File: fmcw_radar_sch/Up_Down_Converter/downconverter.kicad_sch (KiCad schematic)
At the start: 19 parts, among them J11 Conn_Coaxial, J12 Conn_Coaxial, J13 Conn_Coaxial, J14 Conn_01x05_Pin, J6 Conn_Coaxial, U1 ADAR2004ACCZ

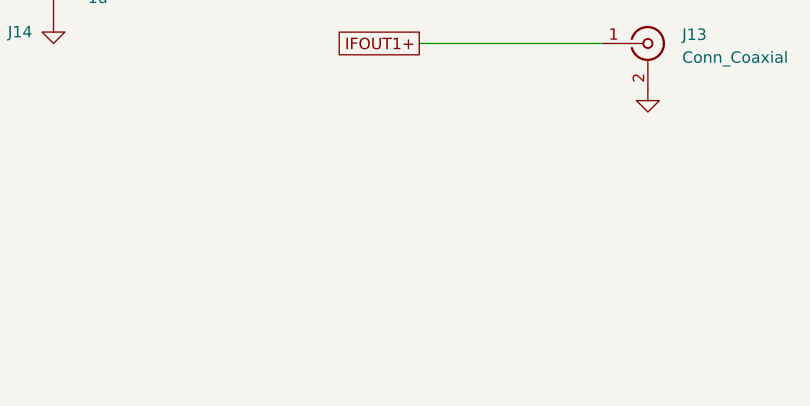
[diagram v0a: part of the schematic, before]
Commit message: changes
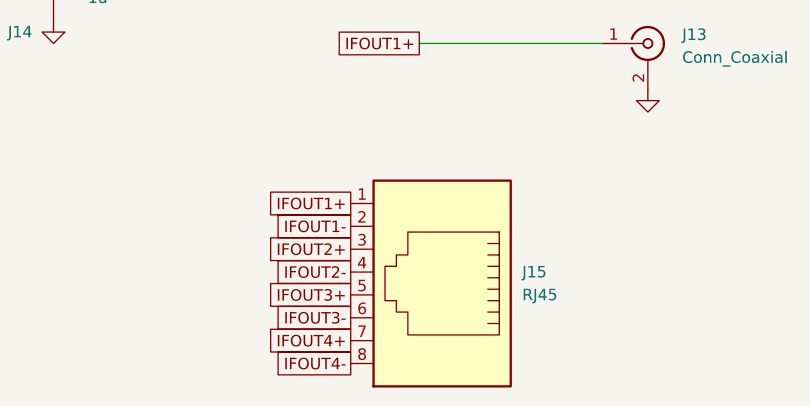
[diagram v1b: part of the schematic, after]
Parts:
- added J15: RJ45, Connector_RJ:RJ45_Amphenol_54602-x08_Horizontal, symbol Connector:RJ45
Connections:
- net IFOUT1+: now also J15.1
- net IFOUT1-: now also J15.2
- net IFOUT2+: now also J15.3
- net IFOUT2-: now also J15.4
- net IFOUT3+: now also J15.5
- net IFOUT3-: now also J15.6
- net IFOUT4+: now also J15.7
- net IFOUT4-: now also J15.8
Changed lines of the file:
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@@
 		)
 	)
+	(global_label "IFOUT4+"
+		(shape passive)
+		(at 208.28 148.59 180)
+		(effects
+			(font
+				(size 1.27 1.27)
+			)
+			(justify right)
+		)
+		(property "Intersheetrefs" "${INTERSHEET_REFS}"
+			(at 208.28 148.59 0)
+			(effects
+				(font
+					(size 1.27 1.27)
+				)
+				(hide yes)
+			)
+		)
+	)
 	(global_label "IFOUT1+"
 		(shape passive)
@@
 		)
 	)
+	(global_label "IFOUT1-"
+		(shape passive)
+		(at 208.28 135.89 180)
+		(effects
+			(font
+				(size 1.27 1.27)
+			)
+			(justify right)
+		)
+		(property "Intersheetrefs" "${INTERSHEET_REFS}"
+			(at 208.28 135.89 0)
+			(effects
+				(font
+					(size 1.27 1.27)
+				)
+				(hide yes)
+			)
+		)
+	)
 	(global_label "RFIN3+"
 		(shape passive)
@@
 		)
 	)
+	(global_label "IFOUT4-"
+		(shape passive)
+		(at 208.28 151.13 180)
+		(effects
+			(font
+				(size 1.27 1.27)
+			)
+			(justify right)
+		)
+		(property "Intersheetrefs" "${INTERSHEET_REFS}"
+			(at 208.28 151.13 0)
+			(effects
+				(font
+					(size 1.27 1.27)
+				)
+				(hide yes)
+			)
+		)
+	)
 	(global_label "RFIN2-"
 		(shape passive)
@@
 		)
 	)
+	(global_label "IFOUT2+"
+		(shape passive)
+		(at 208.28 138.43 180)
+		(effects
+			(font
+				(size 1.27 1.27)
+			)
+			(justify right)
+		)
+		(property "Intersheetrefs" "${INTERSHEET_REFS}"
+			(at 208.28 138.43 0)
+			(effects
+				(font
+					(size 1.27 1.27)
+				)
+				(hide yes)
+			)
+		)
+	)
 	(global_label "IFOUT4-"
 		(shape passive)
@@
 		)
 	)
+	(global_label "IFOUT1+"
+		(shape passive)
+		(at 208.28 133.35 180)
+		(effects
+			(font
+				(size 1.27 1.27)
+			)
+			(justify right)
+		)
+		(property "Intersheetrefs" "${INTERSHEET_REFS}"
+			(at 208.28 133.35 0)
+			(effects
+				(font
+					(size 1.27 1.27)
+				)
+				(hide yes)
+			)
+		)
+	)
 	(global_label "IFOUT1-"
 		(shape passive)
@@
 		)
 	)
+	(global_label "IFOUT3+"
+		(shape passive)
+		(at 208.28 143.51 180)
+		(effects
+			(font
+				(size 1.27 1.27)
+			)
+			(justify right)
+		)
+		(property "Intersheetrefs" "${INTERSHEET_REFS}"
+			(at 208.28 143.51 0)
+			(effects
+				(font
+					(size 1.27 1.27)
+				)
+				(hide yes)
+			)
+		)
+	)
 	(global_label "RFIN3-"
 		(shape passive)
@@
 		)
 	)
+	(global_label "IFOUT3-"
+		(shape passive)
+		(at 208.28 146.05 180)
+		(effects
+			(font
+				(size 1.27 1.27)
+			)
+			(justify right)
+		)
+		(property "Intersheetrefs" "${INTERSHEET_REFS}"
+			(at 208.28 146.05 0)
+			(effects
+				(font
+					(size 1.27 1.27)
+				)
+				(hide yes)
+			)
+		)
+	)
 	(global_label "IFOUT2-"
 		(shape passive)
@@
 		)
 	)
+	(global_label "IFOUT2-"
+		(shape passive)
+		(at 208.28 140.97 180)
+		(effects
+			(font
+				(size 1.27 1.27)
+			)
+			(justify right)
+		)
+		(property "Intersheetrefs" "${INTERSHEET_REFS}"
+			(at 208.28 140.97 0)
+			(effects
+				(font
+					(size 1.27 1.27)
+				)
+				(hide yes)
+			)
+		)
+	)
 	(global_label "VPOS4R"
 		(shape input)
@@
 					(unit 1)
 				)
+			)
+		)
+	)
+	(symbol
+		(lib_id "Connector:RJ45")
+		(at 218.44 140.97 180)
+		(unit 1)
+		(exclude_from_sim no)
+		(in_bom yes)
+		(on_board yes)
+		(dnp no)
+		(fields_autoplaced yes)
+		(property "Reference" "J15"
+			(at 227.33 140.9699 0)
+			(effects
+				(font
+					(size 1.27 1.27)
+				)
+				(justify right)
+			)
+		)
+		(property "Value" "RJ45"
+			(at 227.33 143.5099 0)
+			(effects
+				(font
+					(size 1.27 1.27)
+				)
+				(justify right)
+			)
+		)
+		(property "Footprint" "Connector_RJ:RJ45_Amphenol_54602-x08_Horizontal"
+			(at 218.44 141.605 90)
+			(effects
+				(font
+					(size 1.27 1.27)
+				)
+				(hide yes)
+			)
+		)
+		(property "Datasheet" "~"
+			(at 218.44 141.605 90)
+			(effects
+				(font
+					(size 1.27 1.27)
+				)
+				(hide yes)
+			)
+		)
+		(property "Description" "RJ connector, 8P8C (8 positions 8 connected)"
+			(at 218.44 140.97 0)
+			(effects
+				(font
+					(size 1.27 1.27)
+				)
+				(hide yes)
+			)
+		)
+		(pin "2"
+		)
+		(pin "6"
+		)
+		(pin "8"
+		)
+		(pin "7"
+		)
+		(pin "4"
+		)
+		(pin "1"
+		)
+		(pin "3"
+		)
+		(pin "5"
+		)
+		(instances
+			(project ""
+				(path "/ecdac040-d2fc-4837-bd77-36dd5bdda894/061d5f80-e8b9-4c08-a275-e384bf63be5f"
+					(reference "J15")
+					(unit 1)
+				)

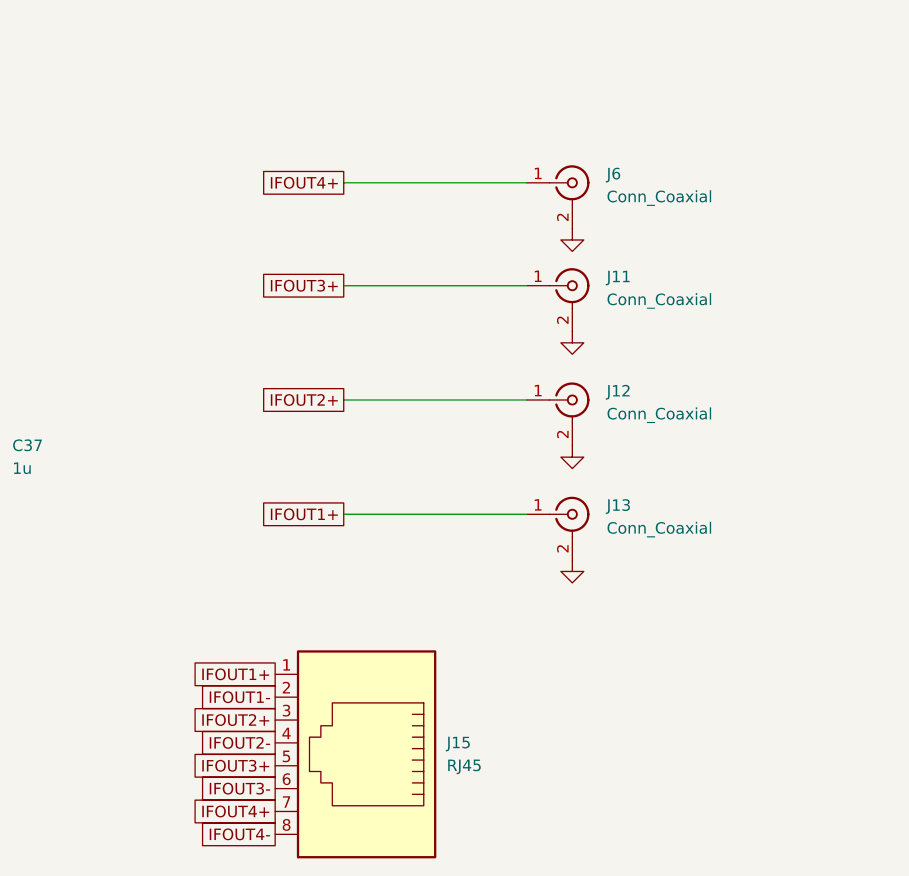
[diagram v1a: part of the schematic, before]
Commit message: a lot of updates
usb power delivery + finishing touches
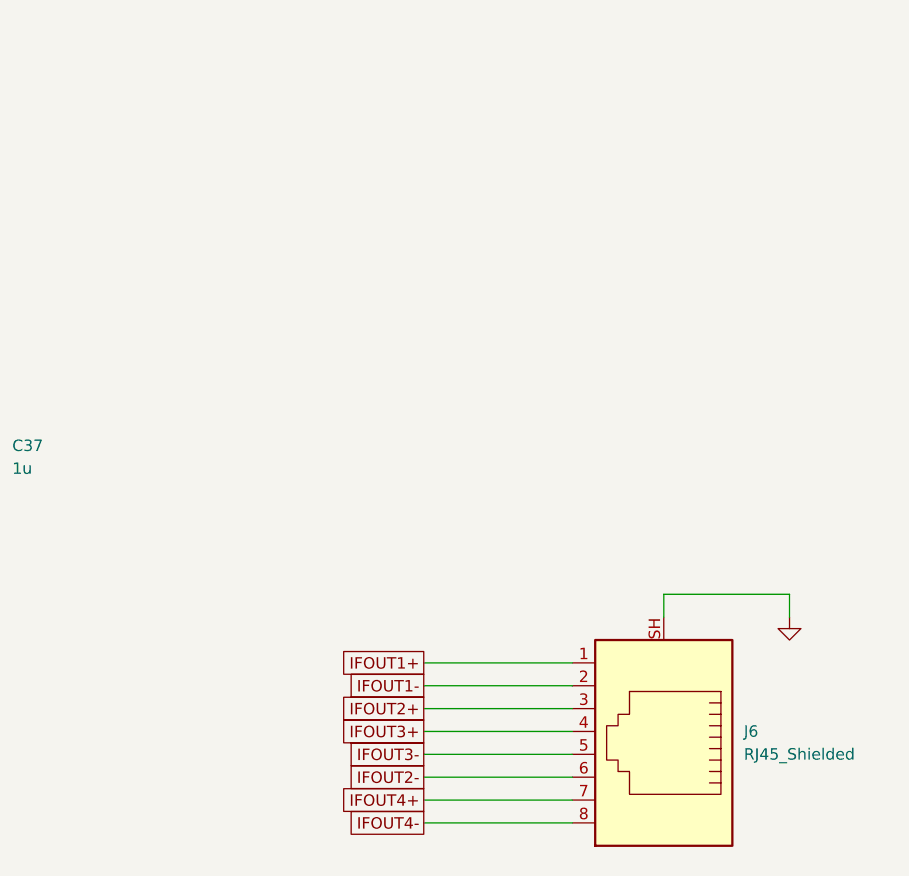
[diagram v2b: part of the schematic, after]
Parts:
- removed J11, J12, J13, J6: Conn_Coaxial, Connector_Coaxial:SMA_Amphenol_132134-10_Vertical, symbol Connector:Conn_Coaxial
- removed J15: RJ45, Connector_RJ:RJ45_Amphenol_54602-x08_Horizontal, symbol Connector:RJ45
- added J6: RJ45_Shielded, symbol Connector:RJ45_Shielded
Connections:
- net GND: now also J6.SH
- net IFOUT1+: now also J6.1
- net IFOUT1-: now also J6.2
- net IFOUT2+: now also J6.3
- net IFOUT2-: now also J6.6
- net IFOUT3+: now also J6.4
- net IFOUT3-: now also J6.5
- net IFOUT4+: now also J6.7
- net IFOUT4-: now also J6.8

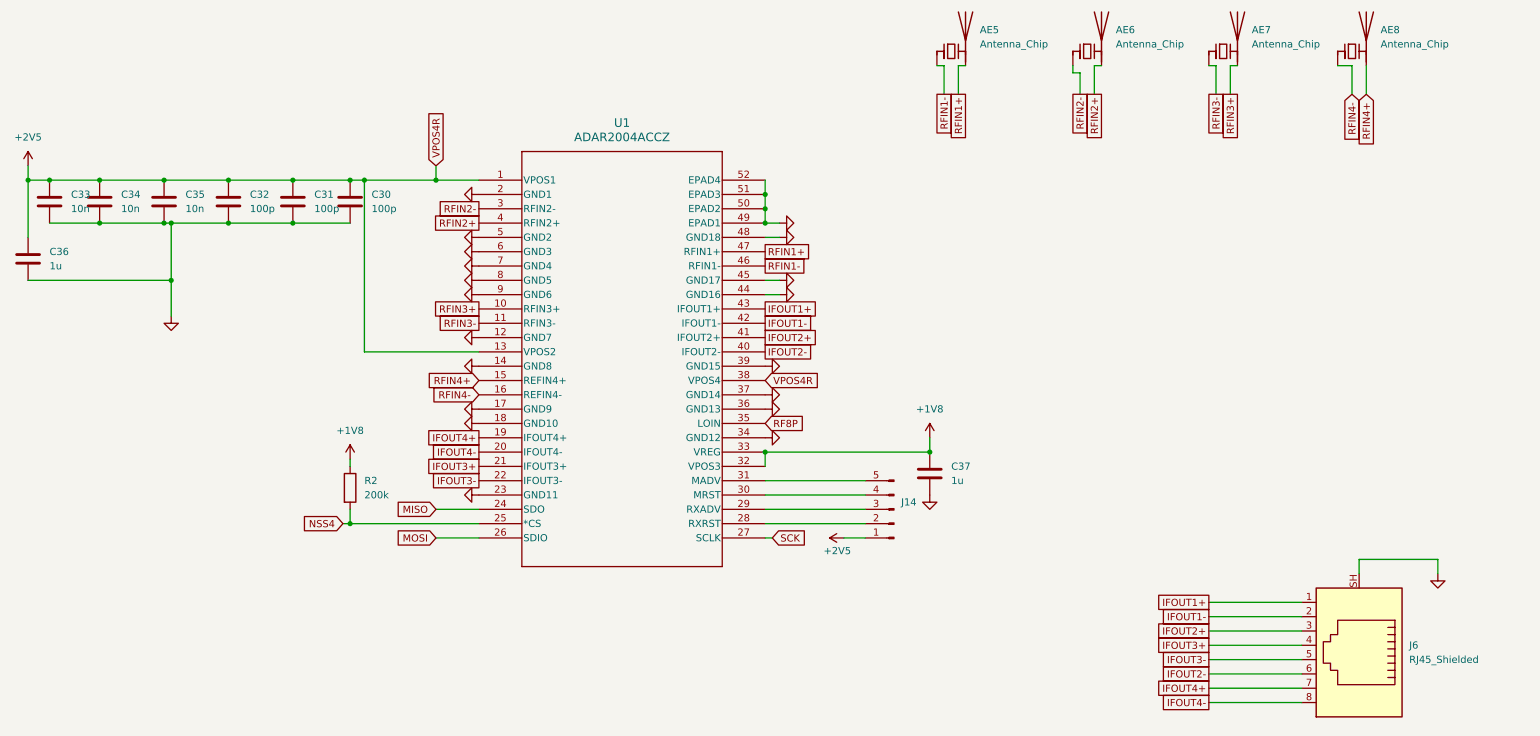
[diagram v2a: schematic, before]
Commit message: Silkscreen finishing
Silkscreen finishting
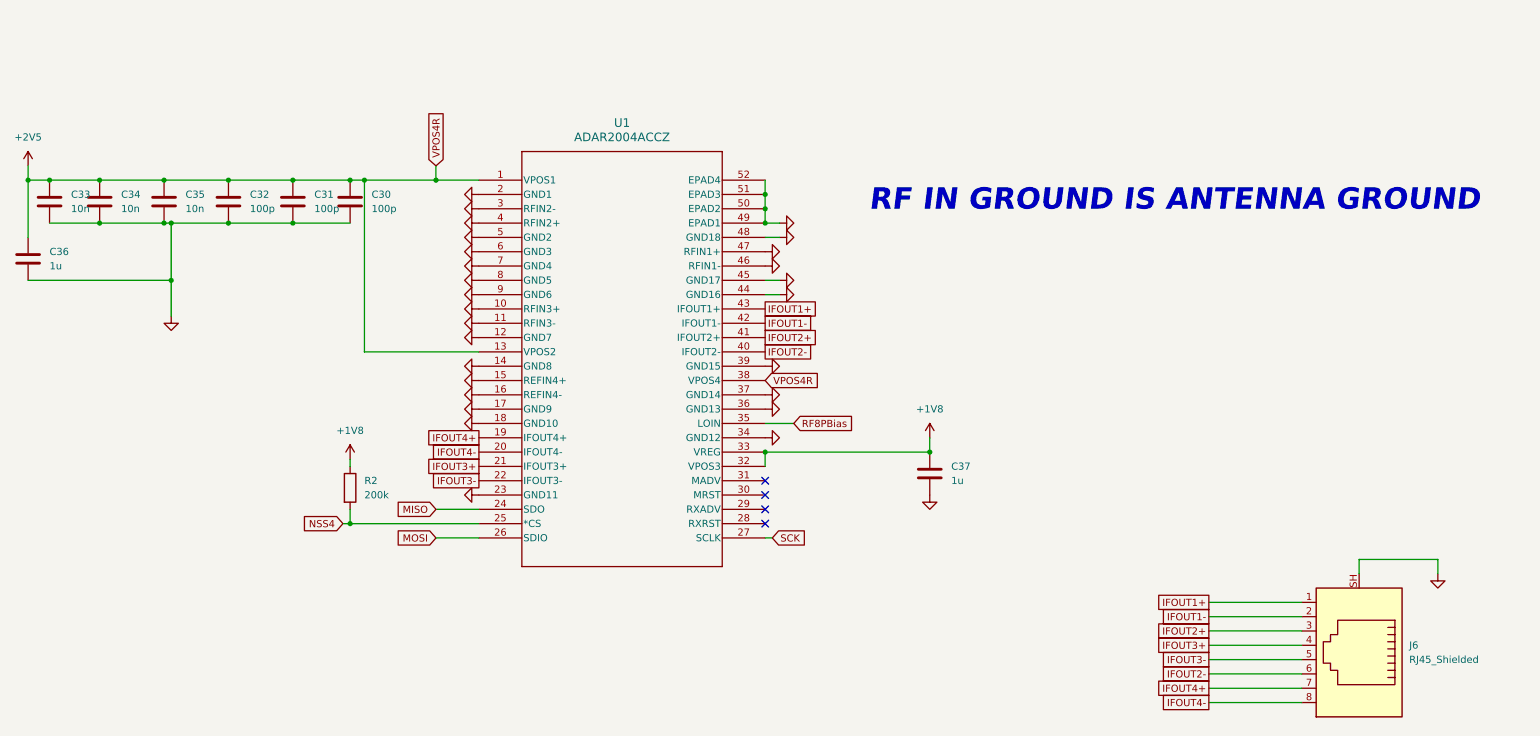
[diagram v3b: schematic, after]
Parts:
- removed AE5, AE6, AE7, AE8: Antenna_Chip, symbol Device:Antenna_Chip
- removed J14: Conn_01x05_Pin, Connector_PinHeader_2.54mm:PinHeader_1x05_P2.54mm_Vertical, symbol Connector:Conn_01x05_Pin
- J6: footprint (none) -> Connector_RJ:RJ45_Amphenol_RJHSE5380
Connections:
- net RFIN1+ is gone; now on net GND: U1.47 (RFIN1+)
- net RFIN1- is gone; now on net GND: U1.46 (RFIN1-)
- net RFIN2+ is gone; now on net GND: U1.4 (RFIN2+)
- net RFIN2- is gone; now on net GND: U1.3 (RFIN2-)
- net RFIN3+ is gone; now on net GND: U1.10 (RFIN3+)
- net RFIN3- is gone; now on net GND: U1.11 (RFIN3-)
- net RFIN4+ is gone; now on net GND: U1.15 (REFIN4+)
- net RFIN4- is gone; now on net GND: U1.16 (REFIN4-)
- net RF8P renamed RF8PBias
- no-connect marks 0 -> 4
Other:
- note added: "RF IN GROUND IS ANTENNA GROUND"
